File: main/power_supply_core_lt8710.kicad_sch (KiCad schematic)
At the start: 33 parts, among them Q301 IXTP28P065T, Q302 TK4R3E06PL, U301 LT8710

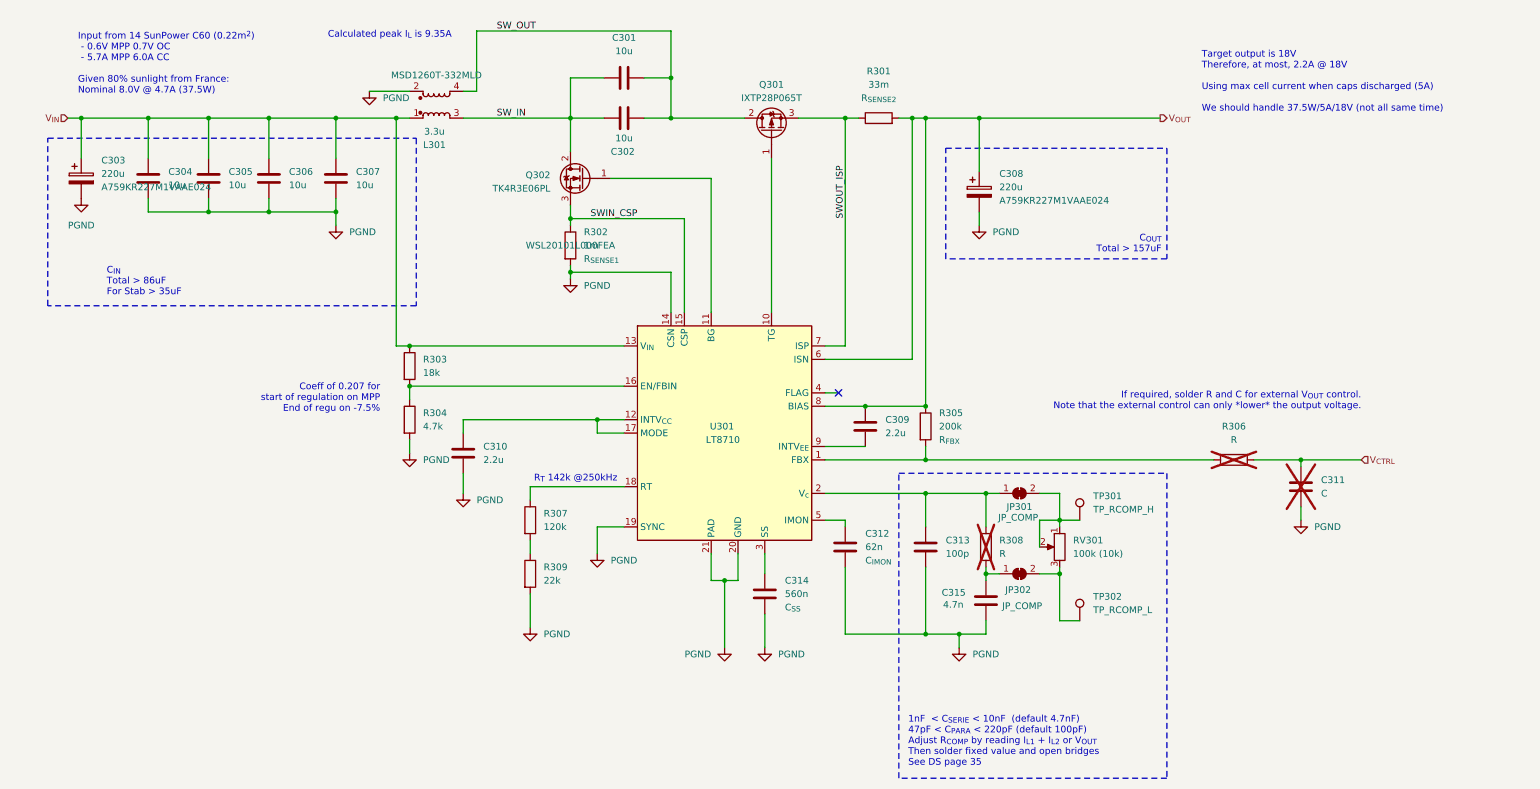
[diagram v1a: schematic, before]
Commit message: Sent to fab
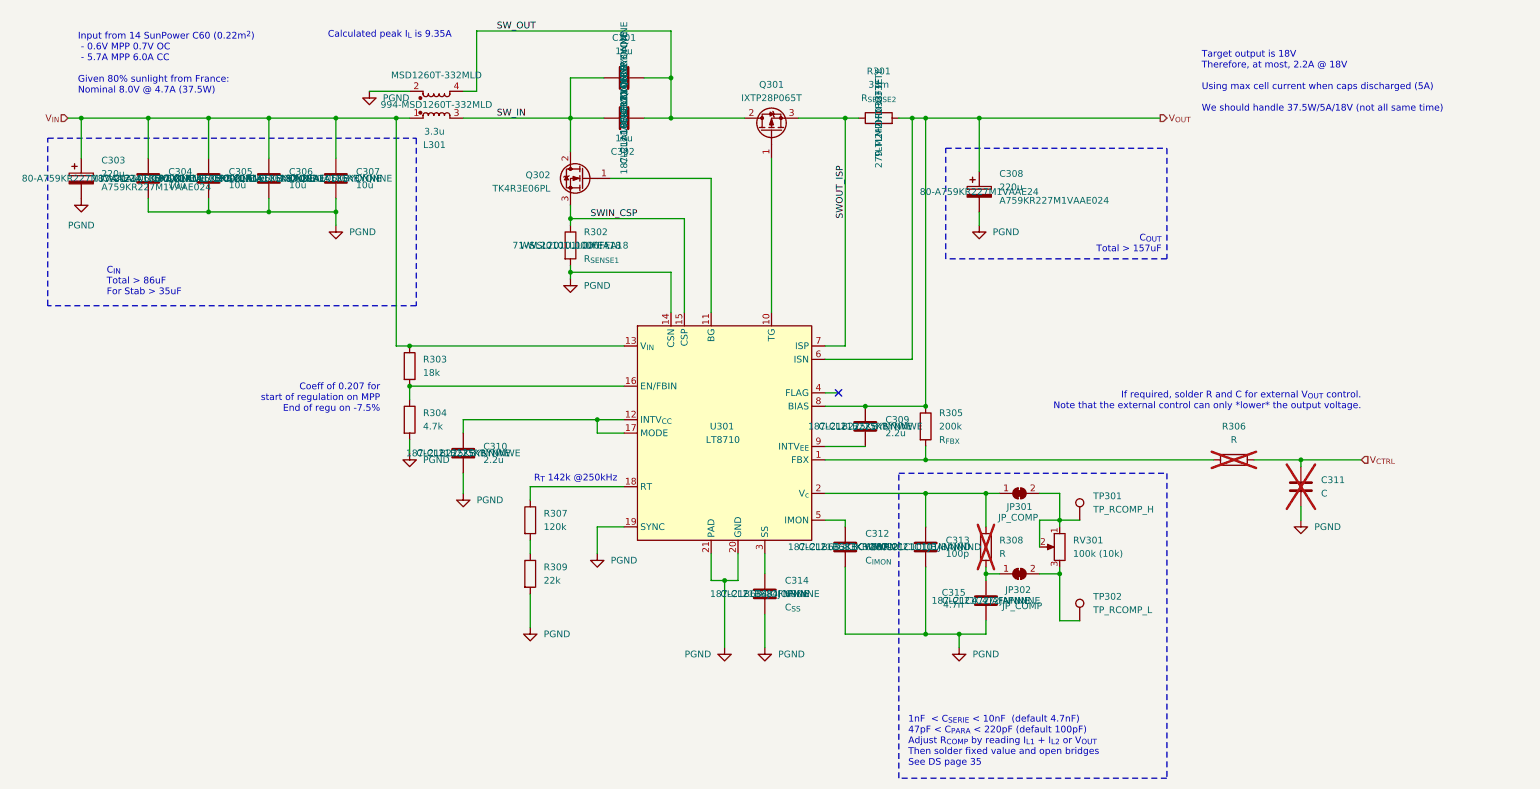
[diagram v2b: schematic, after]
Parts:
- C301, C302, C304, C305, C306, C307: MPN (none) -> CL21A106KBYQNNE; Mouser SKU (none) -> 187-CL21A106KBYQNNE
- C303, C308: Mouser SKU (none) -> 80-A759KR227M1VAAE24
- C309, C310: MPN (none) -> CL21B225KBYNNWE; Mouser SKU (none) -> 187-CL21B225KBYNNWE
- C312: value 62n -> 68n; MPN (none) -> CL21B683KBCWPNC; Mouser SKU (none) -> 187-CL21B683KBCWPNC
- C313: MPN (none) -> CL21C101JBANNND; Mouser SKU (none) -> 187-CL21C101JBANNND
- C314: value 560n -> 680n; MPN (none) -> CL21B684JOFNNNE; Mouser SKU (none) -> 187-CL21B684JOFNNNE
- C315: MPN (none) -> CL21C472JAFNNNE; Mouser SKU (none) -> 187-CL21C472JAFNNNE
- L301: Mouser SKU (none) -> 994-MSD1260T-332MLD
- R301: MPN (none) -> TLM2HDR033FTE; Mouser SKU (none) -> 279-TLM2HDR033FTE
- R302: MPN WSL20101L000FEA -> WSL20101L000FEA18; Mouser SKU (none) -> 71-WSL20101L000FEA18
